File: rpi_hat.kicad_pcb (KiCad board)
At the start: 2 copper layers, 85 x 56 mm, 10 parts, among them U1 RASPBERRY_PI_3_MODEL_B+

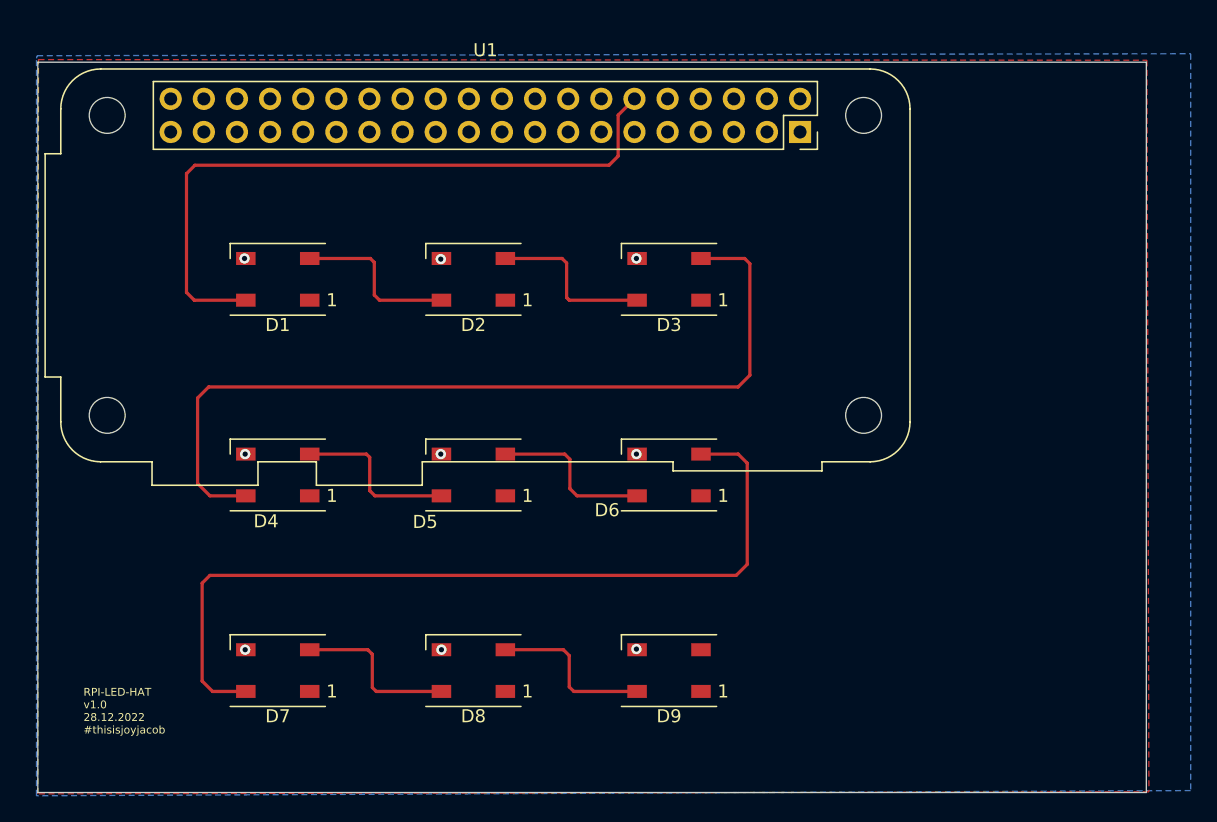
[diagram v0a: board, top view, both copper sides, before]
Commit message: hat changes in design and ideation
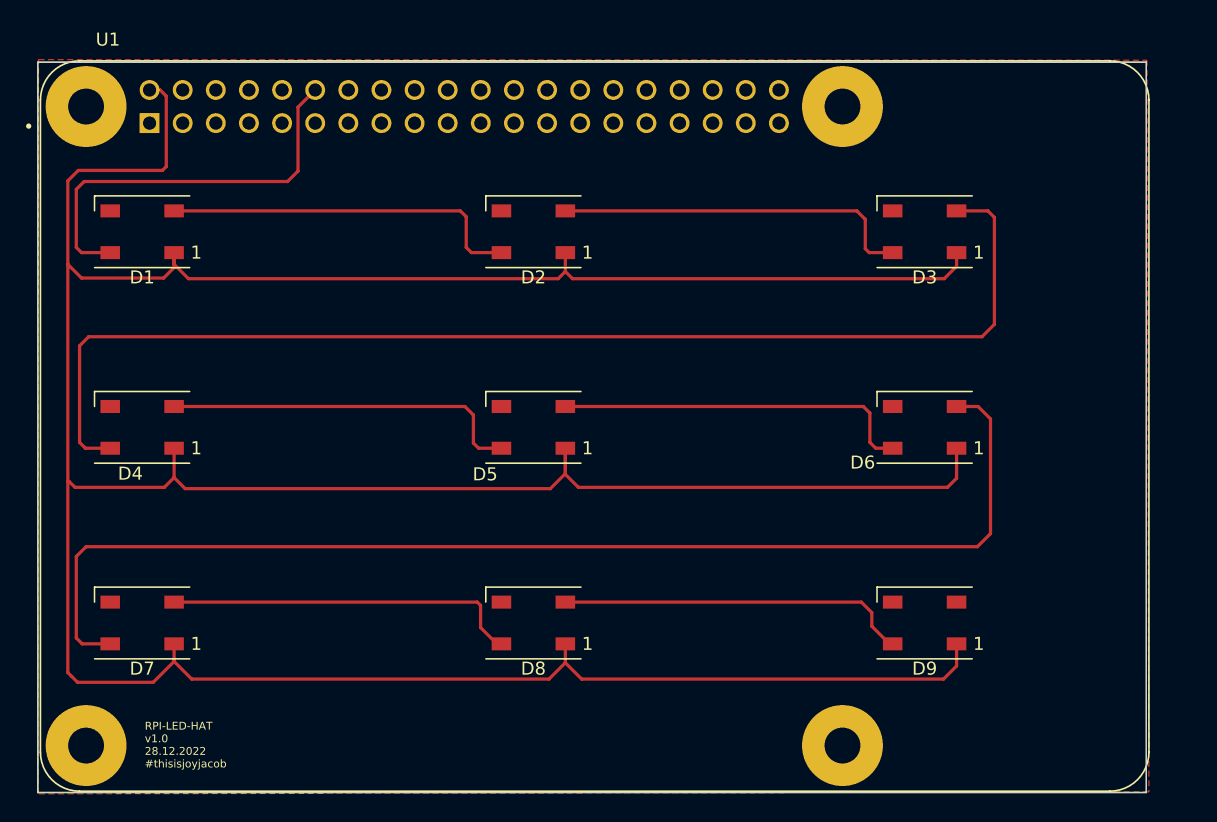
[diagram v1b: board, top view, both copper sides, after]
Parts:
- U1: footprint Module:Raspberry_Pi_Zero_Socketed_THT_FaceDown_MountingHoles -> MODULE_RASPBERRY_PI_3_MODEL_B+:MODULE_RASPBERRY_PI_3_MODEL_B+
- moved U1 27.5 mm to (142.7, 77.9), turned to 0 degrees
- moved D3 19.9 mm to (168.0, 63.0)
- moved D6 19.9 mm to (168.0, 78.0)
- moved D9 19.9 mm to (168.0, 93.0)
- moved D1 11.0 mm to (108.0, 63.0)
- moved D4 11.0 mm to (108.0, 78.0)
- moved D7 11.0 mm to (108.0, 93.0)
- moved D2 5.87 mm to (138.0, 63.0)
- moved D5 5.87 mm to (138.0, 78.0)
- moved D8 5.87 mm to (138.0, 93.0)
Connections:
- D4 pad 1: Net-(D6-Pad1) -> /3v3
- D5 pad 1: Net-(D6-Pad1) -> /3v3
- D6 pad 1: Net-(D6-Pad1) -> /3v3
- D7 pad 1: Net-(D6-Pad1) -> /3v3
- D8 pad 1: Net-(D6-Pad1) -> /3v3
- D9 pad 1: Net-(D6-Pad1) -> /3v3
- U1 pad 1: /3v3 -> Net-(U1-Pad1)
- U1 pad 17: /3v3 -> Net-(U1-Pad1)
- U1 pad 2: Net-(U1-Pad2) -> /3v3
- U1 pad 4: Net-(U1-Pad2) -> /3v3
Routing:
- net /3v3: track 0.00 -> 281.7 mm
- net Net-(D6-Pad2): track 65.2 -> 91.7 mm
- net Net-(D3-Pad2): track 66.2 -> 92.1 mm
- net /RGB: track 52.5 -> 31.6 mm
- net Net-(D5-Pad2): track 12.7 -> 27.7 mm
- net Net-(D1-Pad2): track 12.9 -> 27.8 mm
- net Net-(D2-Pad2): track 13.0 -> 27.7 mm
- net Net-(D4-Pad2): track 12.9 -> 27.7 mm
- net Net-(D7-Pad2): track 12.9 -> 27.4 mm
- net Net-(D8-Pad2): track 12.8 -> 27.0 mm
- net /GND: vias 9 -> 0
- added copper zone on F.Cu, net /GND
- removed copper zone on F.Cu, net /3v3
- removed copper zone on B.Cu, net /GND
